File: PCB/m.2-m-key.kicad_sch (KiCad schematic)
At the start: 16 parts, among them J1 M.2 M-Key Edge Connector

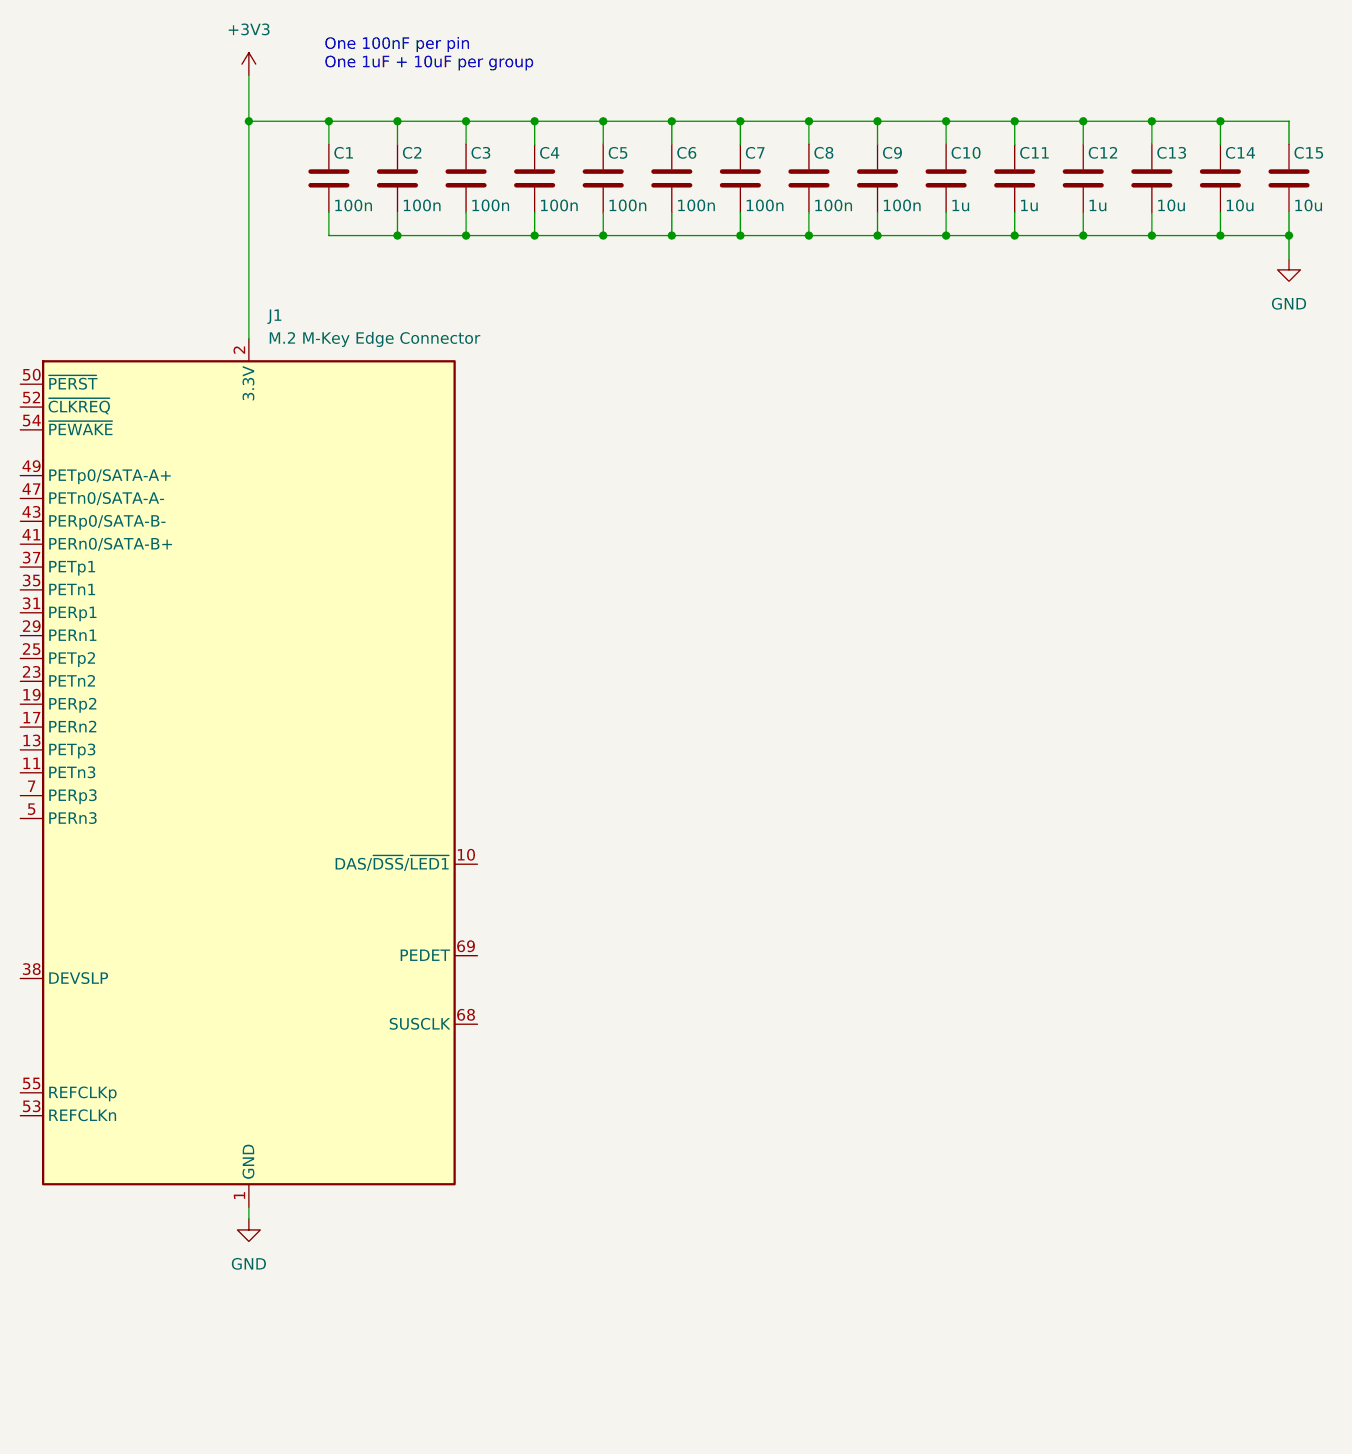
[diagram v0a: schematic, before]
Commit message: fixed JTAGG, working on power architecture
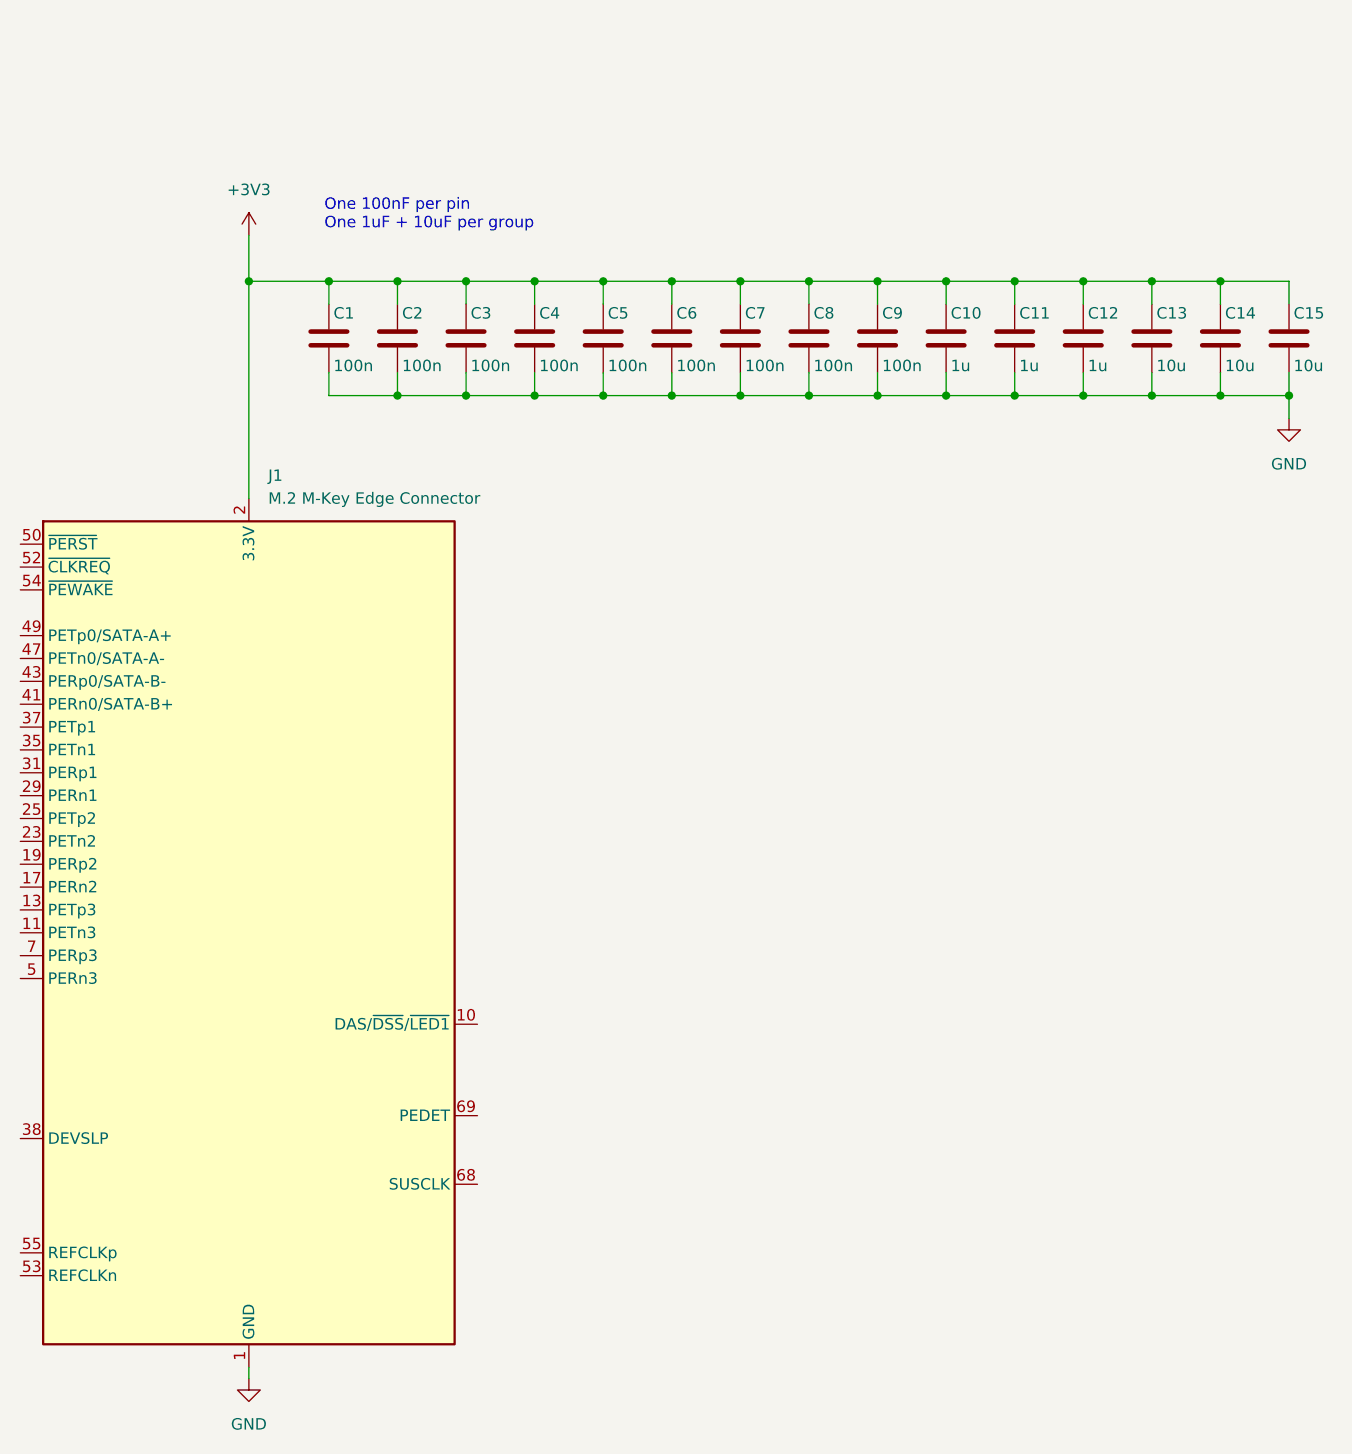
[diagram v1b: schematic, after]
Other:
- moved on the sheet: C1, C10, C11, C12, C13, C14, C15, C2, C3, C4, C5, C6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
